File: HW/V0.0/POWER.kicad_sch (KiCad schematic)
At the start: 50 parts, among them Q10 TVS_2CH, Q3 <name>, Q4 <name>, Q6 <name>, U1 3.3V/300mA, U5 28V/3A Bck

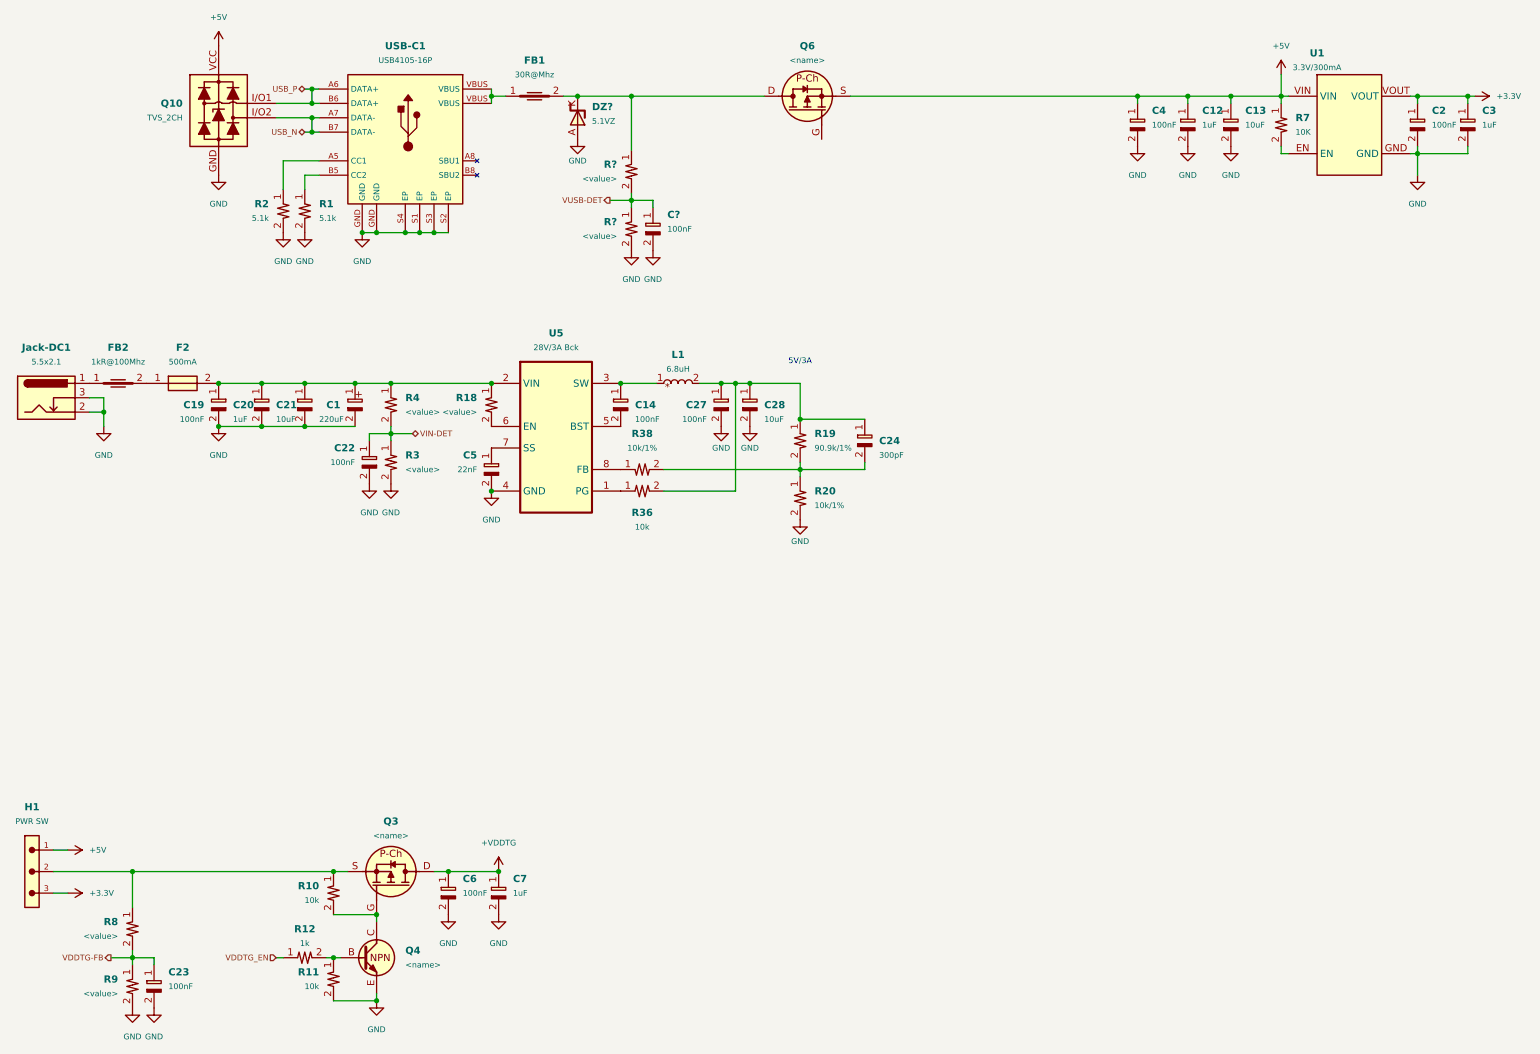
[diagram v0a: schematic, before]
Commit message: PIC16-DevKit-SCH-877 schematic update 4
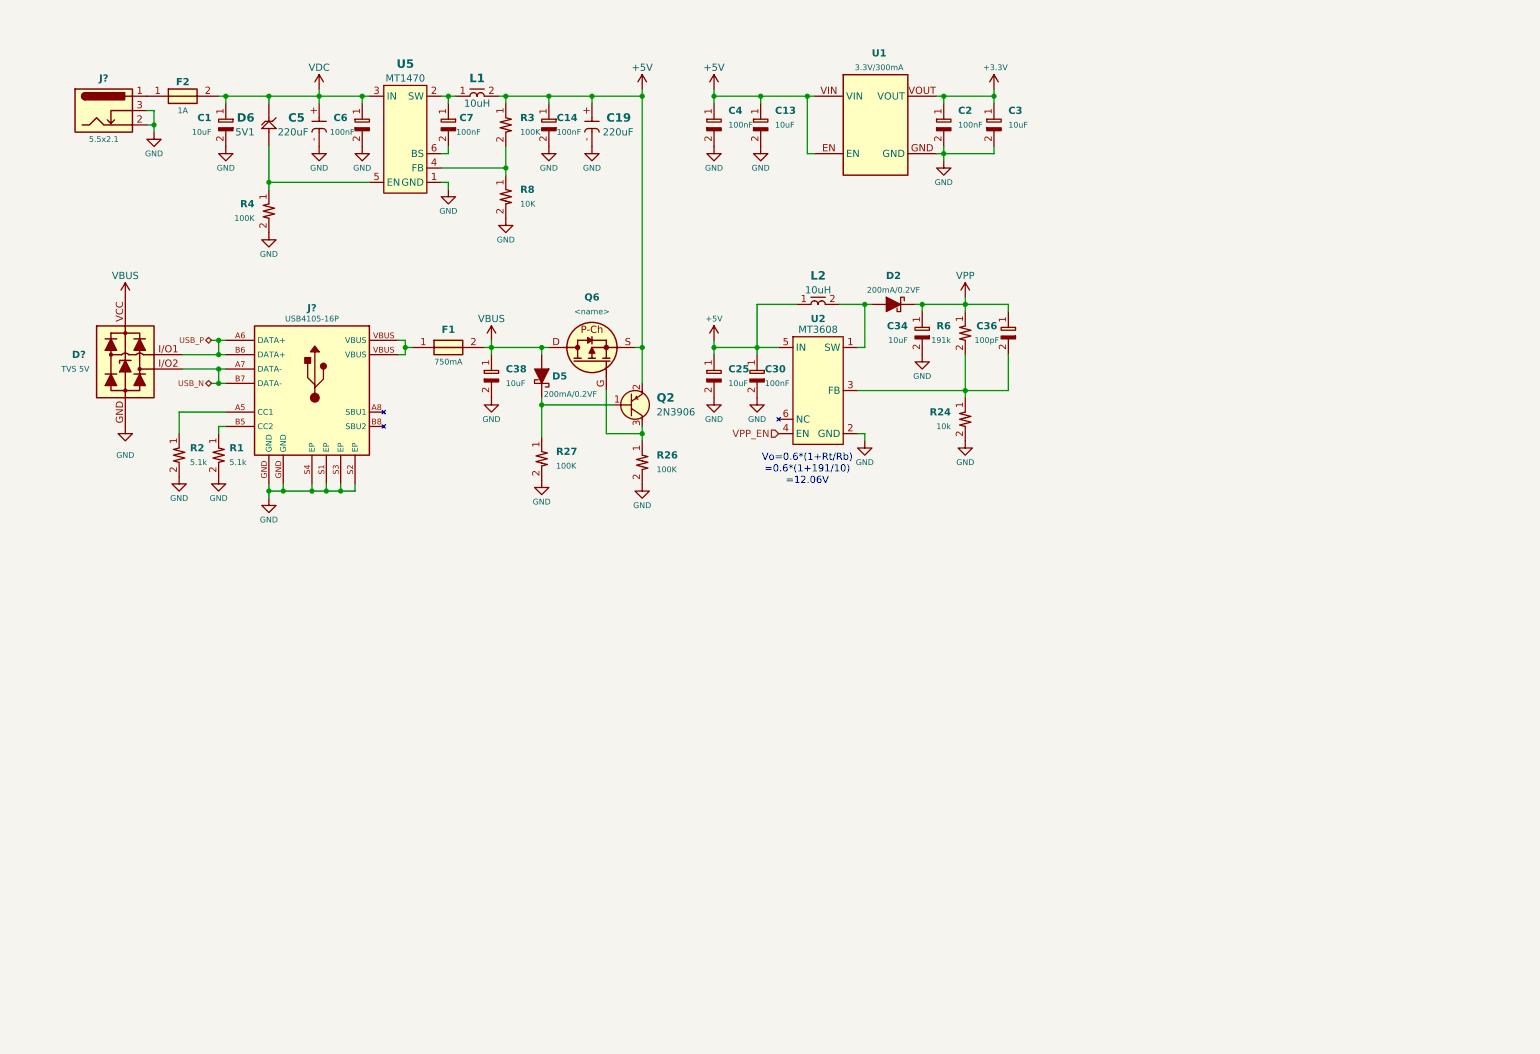
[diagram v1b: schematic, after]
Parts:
- removed C1: 220uF, symbol Triet_KiCAD_Sym:CAP_POL
- removed C12, C20: 1uF, symbol Triet_KiCAD_Sym:CAP_CER
- removed C19, C22, C23, C27, C?: 100nF, symbol Triet_KiCAD_Sym:CAP_CER
- removed C21, C28: 10uF, symbol Triet_KiCAD_Sym:CAP_CER
- removed C24: 300pF, symbol Triet_KiCAD_Sym:CAP_CER
- removed C5: 22nF, symbol Triet_KiCAD_Sym:CAP_CER
- removed DZ?: 5.1VZ, symbol Triet_KiCAD_Sym:Diode ZN
- removed FB1: 30R@Mhz, symbol Triet_KiCAD_Sym: Ferrite Bead
- removed FB2: 1kR@100Mhz, symbol Triet_KiCAD_Sym: Ferrite Bead
- removed H1: PWR SW, Triet_KiCAD_Fprint:Header-3P, symbol Triet_KiCAD_Sym:Header-3P
- removed L1: 6.8uH, symbol Triet_KiCAD_Sym:Ind_Single
- removed Q3: <name>, symbol Triet_KiCAD_Sym:Mosfet-Pch
- removed Q4: <name>, symbol Triet_KiCAD_Sym:NPN
- removed R10, R11, R36: 10k, symbol Triet_KiCAD_Sym:RES
- removed R12: 1k, symbol Triet_KiCAD_Sym:RES
- removed R18, R9, R? (x2): <value>, symbol Triet_KiCAD_Sym:RES
- removed R19: 90.9k/1%, symbol Triet_KiCAD_Sym:RES
- removed R20, R38: 10k/1%, symbol Triet_KiCAD_Sym:RES
- removed R7: 10K, symbol Triet_KiCAD_Sym:RES
- removed U5: 28V/3A Bck, symbol Triet_KiCAD_Sym:MP2338
- added C1, C25, C34, C38: 10uF, symbol Triet_KiCAD_Sym:CAP_CER
- added C19, C5: 220uF, symbol SAMPI:ELECCAP
- added C30: 100nF, symbol Triet_KiCAD_Sym:CAP_CER
- added C36: 100pF, symbol Triet_KiCAD_Sym:CAP_CER
- added D2, D5: 200mA/0.2VF, Liem:SOD-123FL, symbol SAMPI:BAT42
- added D6: 5V1, symbol SAMPI:DIODE-ZEN
- added F1: 750mA, symbol Triet_KiCAD_Sym:Fuse
- added L1, L2: 10uH, symbol SAMPI:IND
- added Q2: 2N3906, SAMPI:SOT23, symbol SAMPI:BJT-PNP
- added R24: 10k, symbol Triet_KiCAD_Sym:RES
- added R26, R27: 100K, symbol Triet_KiCAD_Sym:RES
- added R6: 191k, symbol Triet_KiCAD_Sym:RES
- added U2: MT3608, symbol SAMPI:MT3608
- added U5: MT1470, SAMPI:SOT-23-6_MCHP, symbol SAMPI:MT1470
- C3: value 1uF -> 10uF
- C7: value 1uF -> 100nF
- D?: renamed from Q10; value TVS_2CH -> TVS 5V
- F2: value 500mA -> 1A
- R3, R4: value <value> -> 100K
- R8: value <value> -> 10K
- renumbered USB-C1 to J?, Jack-DC1 to J?
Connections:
- net VDDTG-FB is gone; now on net GND: R8.2
- net +5V: now also C14.1, R3.1, U1.EN, C19.+, C25.1, C30.1, L1.2, L2.1, Q2.2 (E), U2.5 (IN); no longer D?.VCC
- net GND: now also C14.2, R4.2, C1.2, C19.-, C25.2, C30.2, C34.2, C38.2, C5.-, R24.2, R26.2, R27.2, U2.2 (GND), U5.1 (GND); no longer C7.2, R3.2
- net at R8.1: now also R3.2, U5.4 (FB)
- net at R4.1: now also D6.A, U5.5 (EN); no longer F2.2
- net at F2.1: now also J?.1
- net at J?.VBUS: now also F1.1
- net VBUS: now reaches Q6.D
- net VBUS: now also D?.VCC, C38.1, D5.A, F1.2
- net at Q6.G: now also Q2.3 (C), R26.1
- net +VDDTG: no longer names the net of C7.1
- net +VDDTG: now also L1.1, U5.2 (SW); no longer C6.1
- removed net VIN-DET: R3.1, R4.2
- new net: D5.K, Q2.1 (B), R27.1
- new net: D2.A, L2.2, U2.1 (SW)
- new net: C36.2, R24.1, R6.2, U2.3 (FB)
- new net: C7.2, U5.6 (BS)
- new net VDC: C1.1, C5.+, C6.1, D6.K, F2.2, U5.3 (IN)
- new net VPP: C34.1, C36.1, D2.K, R6.1
- new net VPP_EN: U2.4 (EN)
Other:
- note added: "Vo=0.6*(1+Rt/Rb) =0.6*(1+191/10) =12.06V"
- note removed: "5V/3A"
- moved on the sheet: C13, C2, C4, D?, F2, J?, Q6, R1, R2, U1

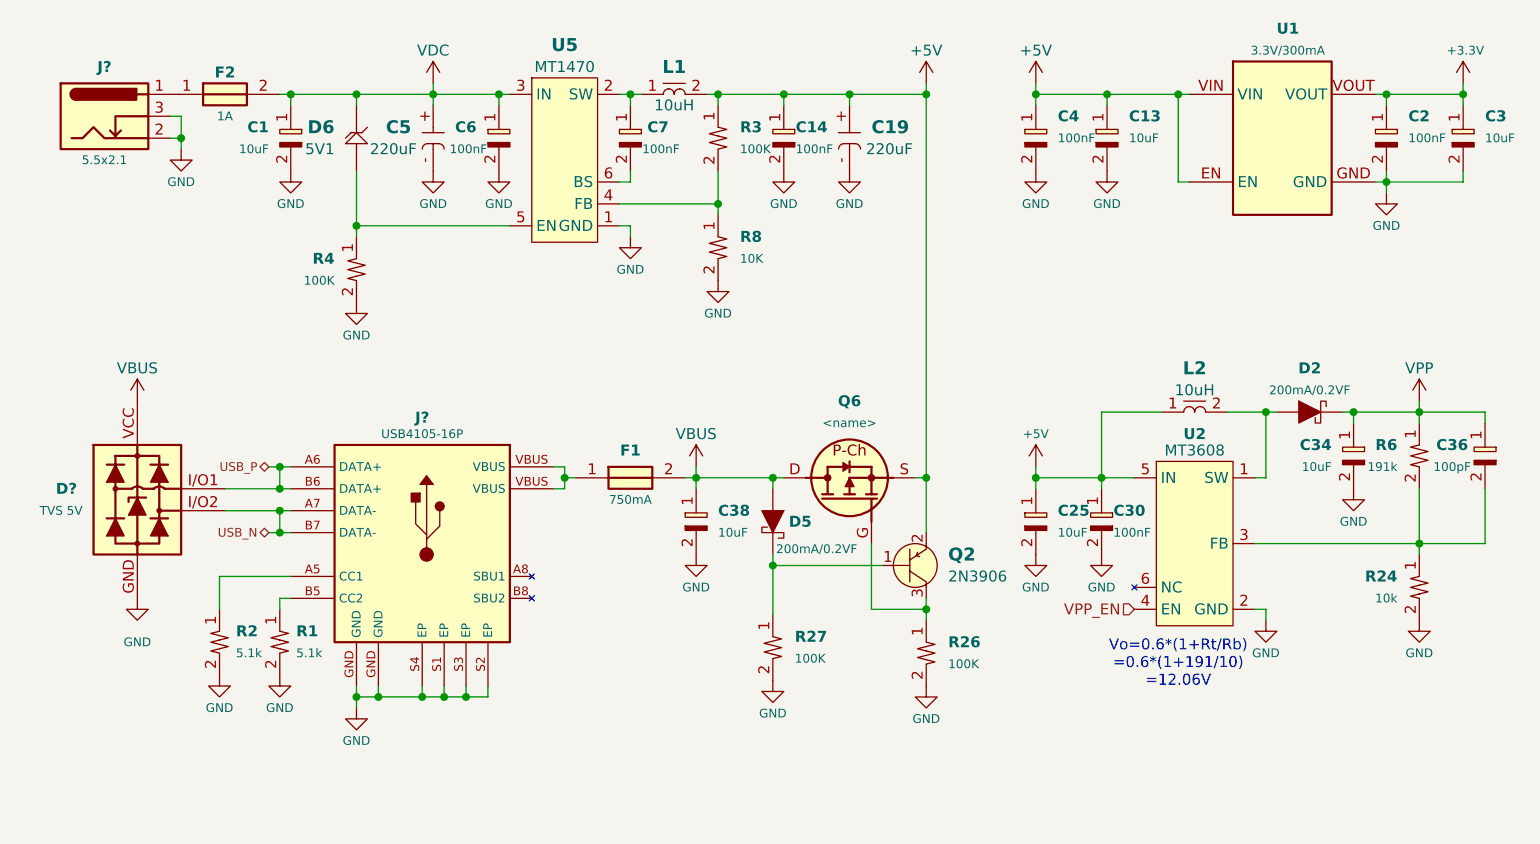
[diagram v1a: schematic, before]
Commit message: PIC16-DevKit-SCH-877 schematic update 5
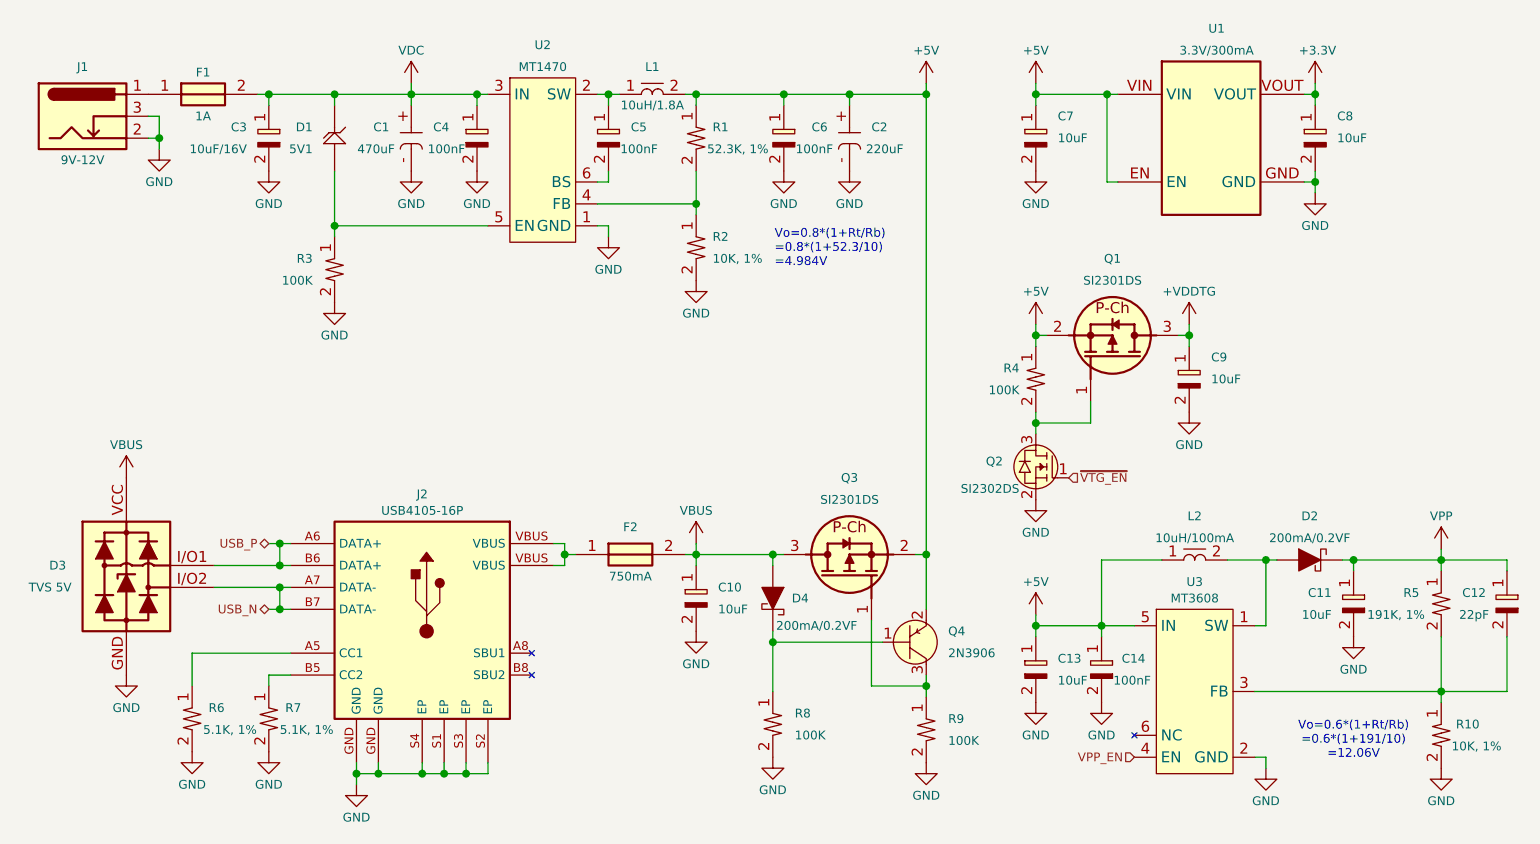
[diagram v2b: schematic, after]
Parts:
- removed C2, C4: 100nF, symbol Triet_KiCAD_Sym:CAP_CER
- added C9: 10uF, SAMPI:CAP0603, symbol Triet_KiCAD_Sym:CAP_CER
- added Q1: SI2301DS, SAMPI:SOT23, symbol Triet_KiCAD_Sym:Mosfet-Pch
- added Q2: SI2302DS, SAMPI:SOT23, symbol SAMPI:FET_N-CH
- added R4: 100K, SAMPI:RES0603, symbol Triet_KiCAD_Sym:RES
- C1: renamed from C5; value 220uF -> 470uF; footprint (none) -> SAMPI:CAP_ELEC-8.3x8.3-DIA8.0
- C10: renamed from C38; footprint (none) -> SAMPI:CAP0603
- C11: renamed from C34; footprint (none) -> SAMPI:CAP0603
- C12: renamed from C36; value 100pF -> 22pF; footprint (none) -> SAMPI:CAP0603
- C13: renamed from C25; footprint (none) -> SAMPI:CAP0603
- C14: renamed from C30; footprint (none) -> SAMPI:CAP0603
- C2: renamed from C19; footprint (none) -> SAMPI:CAP1411
- C3: renamed from C1; value 10uF -> 10uF/16V; footprint (none) -> SAMPI:CAP1206
- C4: renamed from C6; footprint (none) -> SAMPI:CAP0603
- C5: renamed from C7; footprint (none) -> SAMPI:CAP0603
- C6: renamed from C14; footprint (none) -> SAMPI:CAP0603
- C7: renamed from C13; footprint (none) -> SAMPI:CAP0603
- C8: renamed from C3; footprint (none) -> SAMPI:CAP0603
- D1: renamed from D6; footprint (none) -> SAMPI:SOD80C-LL34
- D3: renamed from D?; MPN PRTR5V0U2X,215 -> (none)
- F1: renamed from F2; footprint (none) -> SAMPI:FUSE1812
- F2: renamed from F1; footprint (none) -> SAMPI:FUSE1812
- J1: renamed from J?; value 5.5x2.1 -> 9V-12V
- J2: renamed from J?; MPN USB4105-GF-A -> (none)
- L1: value 10uH -> 10uH/1.8A; footprint (none) -> SAMPI:IND5852
- L2: value 10uH -> 10uH/100mA; footprint (none) -> SAMPI:IND0805
- Q3: renamed from Q6; value <name> -> SI2301DS; footprint (none) -> SAMPI:SOT23
- R1: renamed from R3; value 100K -> 52.3K, 1%; footprint (none) -> SAMPI:RES0603
- R10: renamed from R24; value 10k -> 10K, 1%; footprint (none) -> SAMPI:RES0603
- R2: renamed from R8; value 10K -> 10K, 1%; footprint (none) -> SAMPI:RES0603
- R3: renamed from R4; footprint (none) -> SAMPI:RES0603
- R5: renamed from R6; value 191k -> 191K, 1%; footprint (none) -> SAMPI:RES0603
- R6: renamed from R2; value 5.1k -> 5.1K, 1%; footprint (none) -> SAMPI:RES0603
- R7: renamed from R1; value 5.1k -> 5.1K, 1%; footprint (none) -> SAMPI:RES0603
- R8: renamed from R27; footprint (none) -> SAMPI:RES0603
- R9: renamed from R26; footprint (none) -> SAMPI:RES0603
- U1: MPN MIC5504-3.3YM5-TR -> (none)
- U3: renamed from U2; footprint (none) -> SAMPI:SOT-23-6_MCHP
- renumbered D5 to D4, Q2 to Q4, U5 to U2
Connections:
- net +5V: now also Q3.2 (S), Q1.2 (S), R4.1; no longer Q3.S
- net GND: now also C9.2, Q2.2 (S)
- net VBUS: now also Q3.3 (D); no longer Q3.D
- net at Q4.3 (C), R9.1: now also Q3.1 (G); no longer Q3.G
- new net: Q1.1 (G), Q2.3 (D), R4.2
- new net +VDDTG: C9.1, Q1.3 (D)
- new net ~{VTG_EN}: Q2.1 (G)
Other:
- moved on the sheet: C1, C10, C11, C12, C13, C14, C3, C4, C5, C7, C8, D1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
